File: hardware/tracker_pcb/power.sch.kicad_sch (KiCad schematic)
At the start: 13 parts, among them U2 TPS62933FDRLR

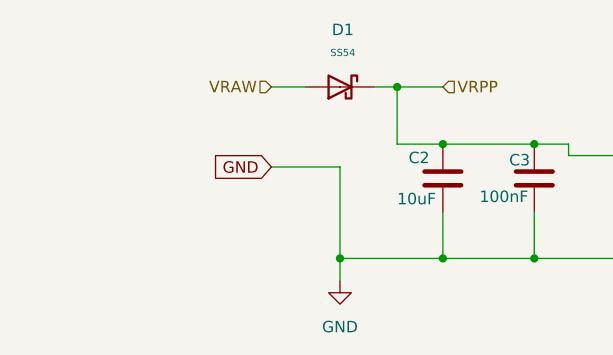
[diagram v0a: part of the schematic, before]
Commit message: WIP
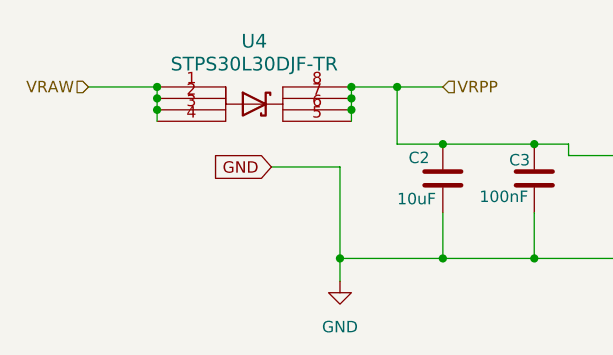
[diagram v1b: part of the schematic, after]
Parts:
- removed D1: SS54, Diode_SMD:D_SMA, symbol PCM_JLCPCB-Diodes:Schottky,SS54
- added U4: STPS30L30DJF-TR, footprint:SON_0L30DJF-TR_STM, symbol symbol:STPS30L30DJF-TR
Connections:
- net VRAW: now also U4.1, U4.2, U4.3, U4.4
- net VRPP: now also U4.5, U4.6, U4.7, U4.8

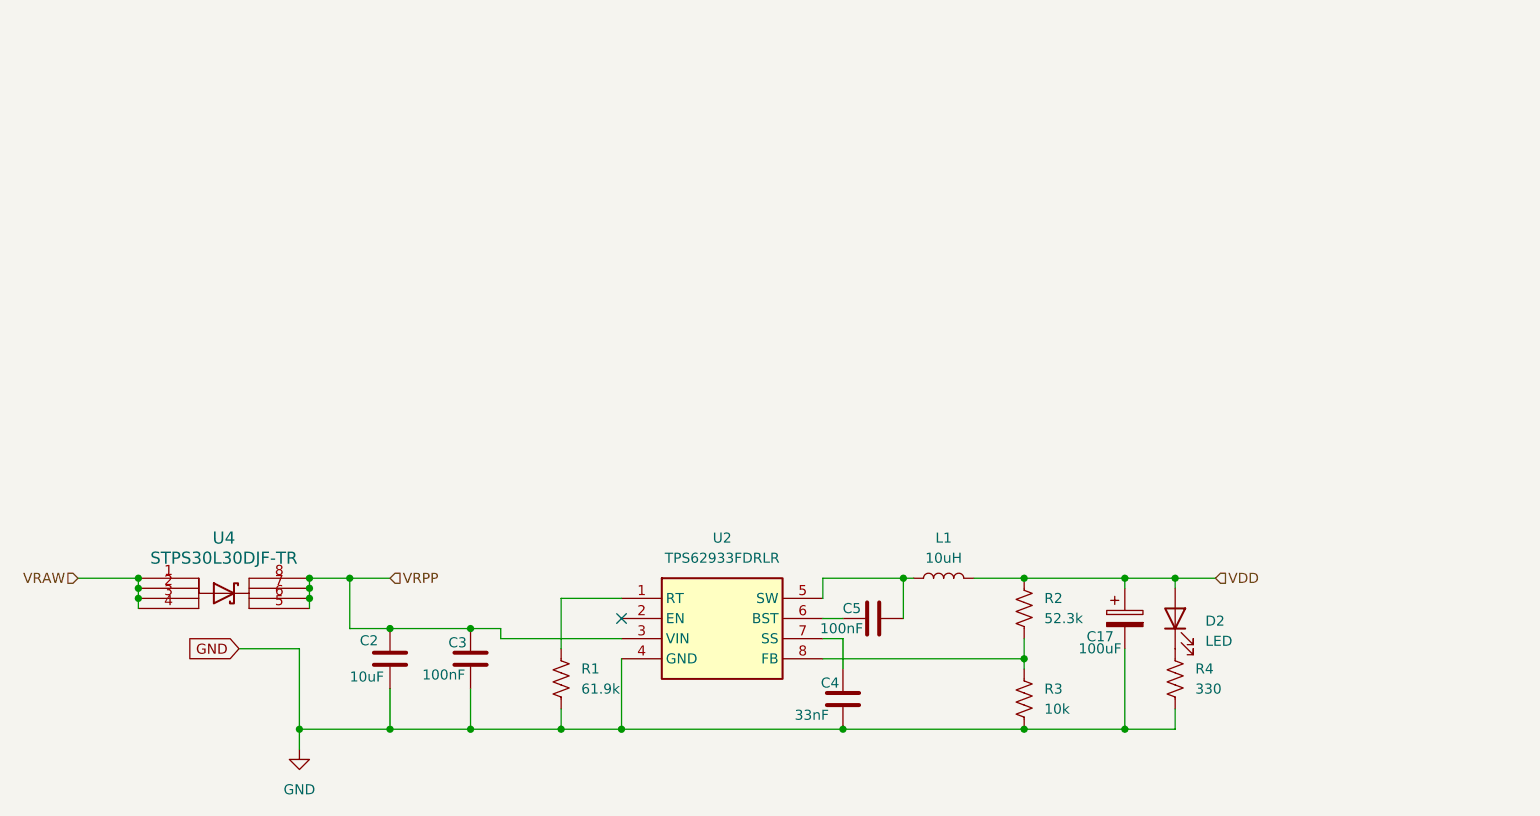
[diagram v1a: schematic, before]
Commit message: Including LORA wio-sx1262
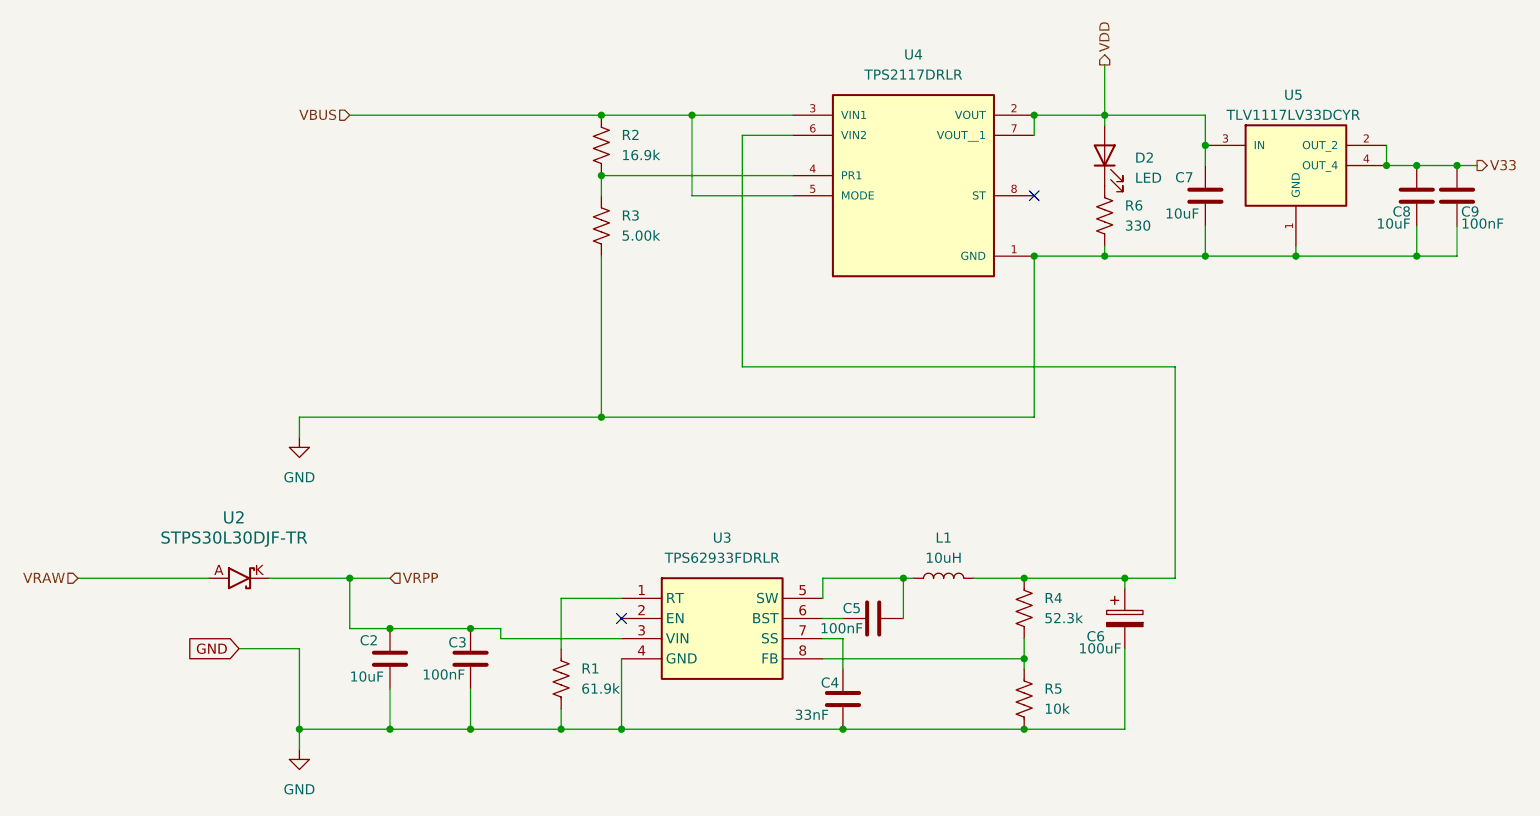
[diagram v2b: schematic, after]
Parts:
- added C7, C8: 10uF, Capacitor_SMD:C_1206_3216Metric, symbol Device:C
- added C9: 100nF, Capacitor_SMD:C_0603_1608Metric, symbol Device:C
- added R2: 16.9k, Resistor_SMD:R_0603_1608Metric, symbol Device:R_US
- added R3: 5.00k, Resistor_SMD:R_0603_1608Metric, symbol Device:R_US
- added U4: TPS2117DRLR, footprint:SOTFL50P160X60-8N, symbol symbol:TPS2117DRLR
- added U5: TLV1117LV33DCYR, footprint:VREG_TLV1117LV33DCYR, symbol symbol:TLV1117LV33DCYR
- C2: LCSC (none) -> C1849
- C3, C5: LCSC (none) -> C1590
- C4: LCSC (none) -> C1614
- C6: renamed from C17; LCSC (none) -> C59944
- D2: LCSC (none) -> C12624
- L1: LCSC (none) -> C526017
- R1: LCSC (none) -> C23091
- R4: renamed from R2; LCSC (none) -> C185323
- R5: renamed from R3; LCSC (none) -> C25804
- R6: renamed from R4; LCSC (none) -> C23138
- U3: renamed from U2; LCSC (none) -> C5219272
- renumbered U4 to U2
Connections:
- net GND: now also C7.2, C8.2, C9.2, R3.1, U4.1 (GND), U5.1 (GND)
- net VDD: now also C7.1, U4.2 (VOUT), U4.7 (VOUT__1), U5.3 (IN); no longer C6.1, L1.2, R4.2
- net VRAW: now also U2.A; no longer U2.1, U2.2, U2.3, U2.4
- net VRPP: now also U2.K; no longer U2.5, U2.6, U2.7, U2.8
- new net: R2.1, R3.2, U4.4 (PR1)
- new net: C6.1, L1.2, R4.2, U4.6 (VIN2)
- new net V33: C8.1, C9.1, U5.2 (OUT_2), U5.4 (OUT_4)
- new net VBUS: R2.2, U4.3 (VIN1), U4.5 (MODE)
- no-connect marks 1 -> 2
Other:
- moved on the sheet: D2, R6
